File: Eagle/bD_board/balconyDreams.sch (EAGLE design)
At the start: 35 parts, among them IC1 7805L, Q1 2N7002, Q2 2N7002, Q3 2N7002, Q4 2N7002, Q5 2N7002, Q6 2N7002, Q7 2N7002, Q8 2N7002, U1 MKR1000, X2 MKDSN1,5/2-5,08

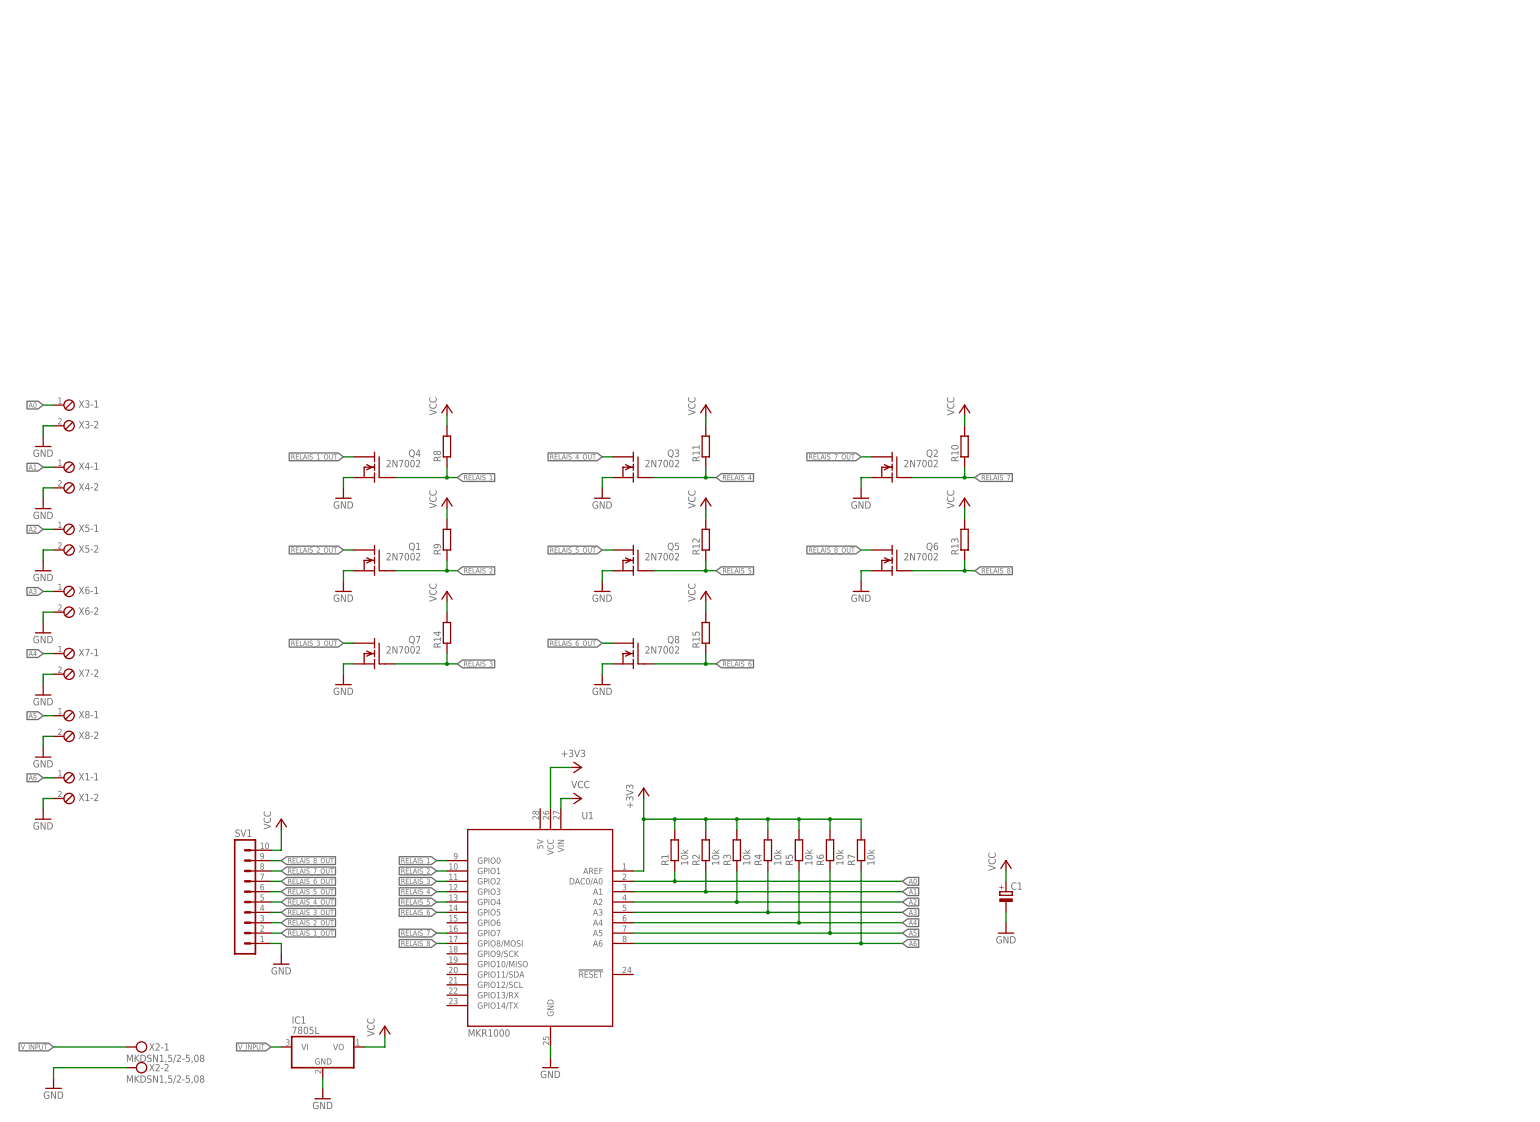
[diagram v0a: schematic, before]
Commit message: Lots of stuff - ready for review
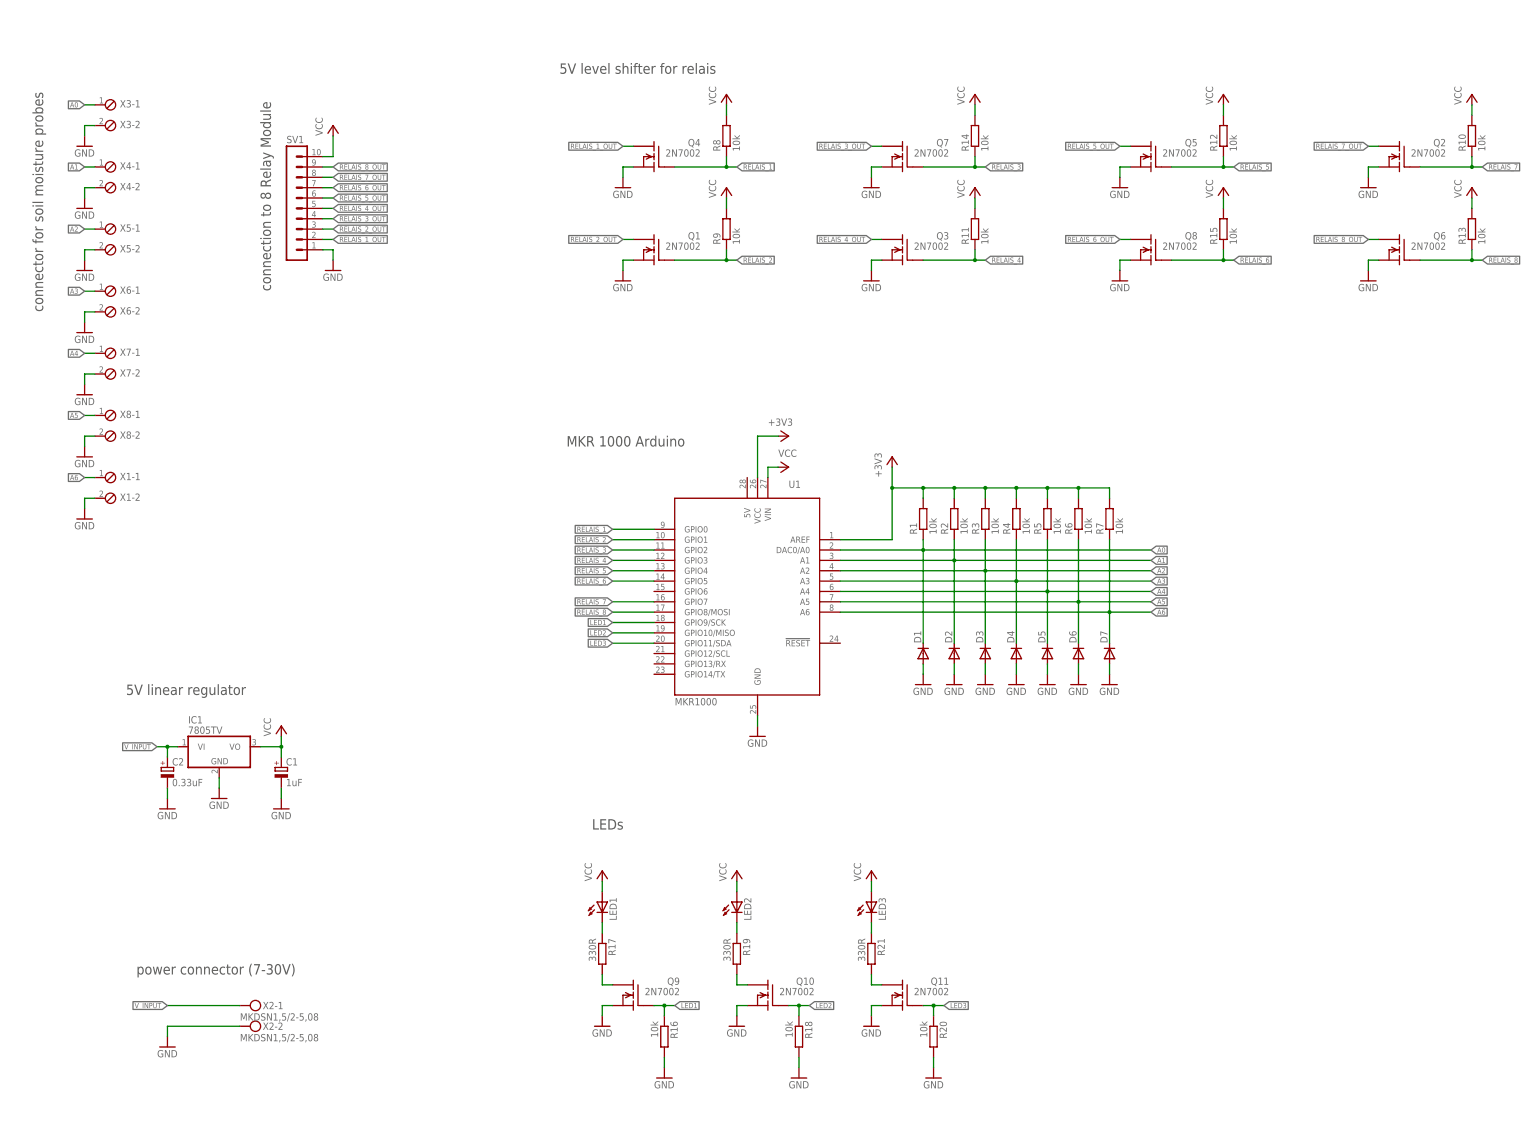
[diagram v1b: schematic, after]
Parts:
- added C2: 0.33uF, rcl:CPOL-EUE5-6
- added D1, D2, D3, D4, D5, D6, D7: (no value), diode:DIODE-SOD323-W
- added LED1, LED2, LED3: (no value), led:LEDCHIPLED_0805
- added Q10, Q11, Q9: 2N7002, transistors_gaui:2N7002
- added R16, R18, R20: 10k, rcl:R-EU_R0805
- added R17, R19, R21: 330R, rcl:R-EU_R0805
- C1: value (none) -> 1uF
- IC1: value 7805L -> 7805TV; device linear:7805L -> linear:7805TV
- R10, R11, R12, R13, R14, R15, R8, R9: value (none) -> 10k
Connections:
- new net LED1: Q9.G, R16.1, U1.GPIO9/SCK
- new net LED2: Q10.G, R18.1, U1.GPIO10/MISO
- new net LED3: Q11.G, R20.1, U1.GPIO11/SDA
- new net N$1: LED1.C, R17.1
- new net N$2: Q9.D, R17.2
- new net N$3: Q10.D, R19.2
- new net N$4: LED2.C, R19.1
- new net N$5: Q11.D, R21.2
- new net N$6: LED3.C, R21.1
- net A0: now also D1.C
- net A1: now also D2.C
- net A2: now also D3.C
- net A3: now also D4.C
- net A4: now also D5.C
- net A5: now also D6.C
- net A6: now also D7.C
- net GND: now also C2.-, D1.A, D2.A, D3.A, D4.A, D5.A, D6.A, D7.A, Q10.S, Q11.S, Q9.S, R16.2, R18.2, R20.2
- net VCC: now also LED1.A, LED2.A, LED3.A
- net V_INPUT: now also C2.+
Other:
- note added: "5V level shifter for relais"
- note added: "5V linear regulator"
- note added: "LEDs"
- note added: "MKR 1000 Arduino"
- note added: "connection to 8 Relay Module"
- note added: "connector for soil moisture probes"
- note added: "power connector (7-30V)"
- moved on the sheet: C1, IC1, Q1, Q2, Q3, Q4, Q5, Q6, Q7, Q8, R1, R10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
